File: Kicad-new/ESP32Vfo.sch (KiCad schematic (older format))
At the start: 63 parts, among them J1 ILI9341, J2 5V, J3 Jtag, J4 I2C, J6 I2C, J7 Encoders, J8 Encoders, J9 Analog in 3-6, SW1 SW_Push, SW2 SW_Push, U1 LM1117-3.3, U2 ESP32-WROOM-32D, U3 PCF8574A, U5 TCA9548APWR

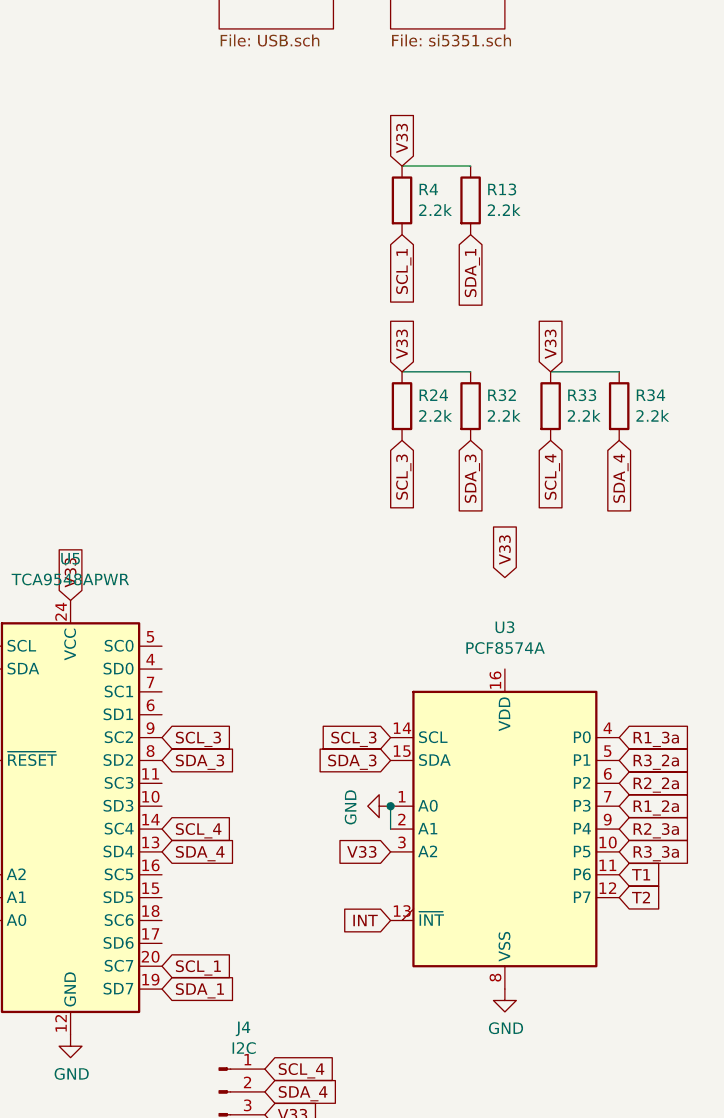
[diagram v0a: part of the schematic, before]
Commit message: new pcb
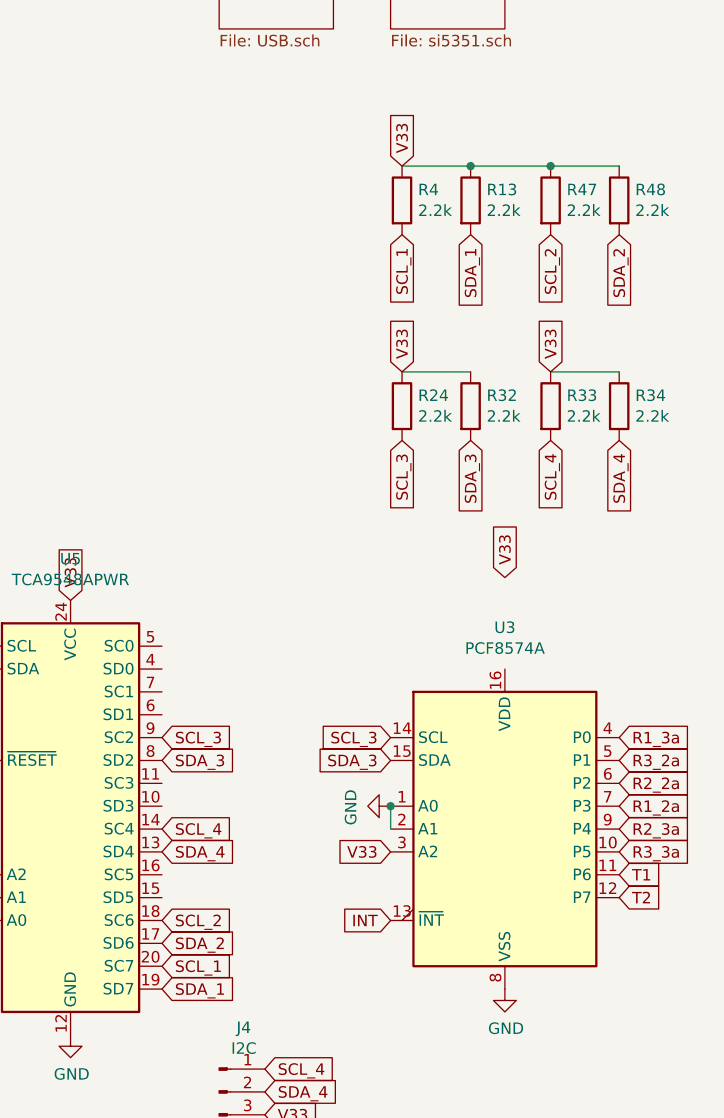
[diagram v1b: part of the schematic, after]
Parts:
- added R47, R48: 2.2k, Resistor_SMD:R_0805_2012Metric, symbol Device:R
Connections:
- net V33: now also R47.1, R48.1
- net SDA_2: now reaches U5.17 (SD6)
- net SDA_2: now also R48.2
- net SCL_2: now reaches U5.18 (SC6)
- net SCL_2: now also R47.2
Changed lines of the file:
@@
 Wire Wire Line
 	2050 1800 2300 1800
+Text GLabel 8850 5050 2    50   Input ~ 0
+SCL_2
+Text GLabel 8850 5150 2    50   Input ~ 0
+SDA_2
+$Comp
+L Device:R R?
+U 1 1 6169519F
+P 10550 1900
+AR Path="/614F5619/6169519F" Ref="R?"  Part="1"
+AR Path="/61506CC0/6169519F" Ref="R?"  Part="1"
+AR Path="/6169519F" Ref="R47"  Part="1"
+F 0 "R47" H 10620 1946 50  0000 L CNN
+F 1 "2.2k" H 10620 1855 50  0000 L CNN
+F 2 "Resistor_SMD:R_0805_2012Metric" V 10480 1900 50  0001 C CNN
+F 3 "~" H 10550 1900 50  0001 C CNN
+	1    10550 1900
+	1    0    0    -1
+$EndComp
+$Comp
+L Device:R R?
+U 1 1 616958E1
+P 10850 1900
+AR Path="/614F5619/616958E1" Ref="R?"  Part="1"
+AR Path="/61506CC0/616958E1" Ref="R?"  Part="1"
+AR Path="/616958E1" Ref="R48"  Part="1"
+F 0 "R48" H 10920 1946 50  0000 L CNN
+F 1 "2.2k" H 10920 1855 50  0000 L CNN
+F 2 "Resistor_SMD:R_0805_2012Metric" V 10780 1900 50  0001 C CNN
+F 3 "~" H 10850 1900 50  0001 C CNN
+	1    10850 1900
+	1    0    0    -1
+$EndComp
+Text GLabel 10550 2050 3    50   Input ~ 0
+SCL_2
+Text GLabel 10850 2050 3    50   Input ~ 0
+SDA_2
+Wire Wire Line
+	10200 1750 10550 1750
+Connection ~ 10200 1750
+Connection ~ 10550 1750
+Wire Wire Line
+	10550 1750 10850 1750
 $EndSCHEMATC

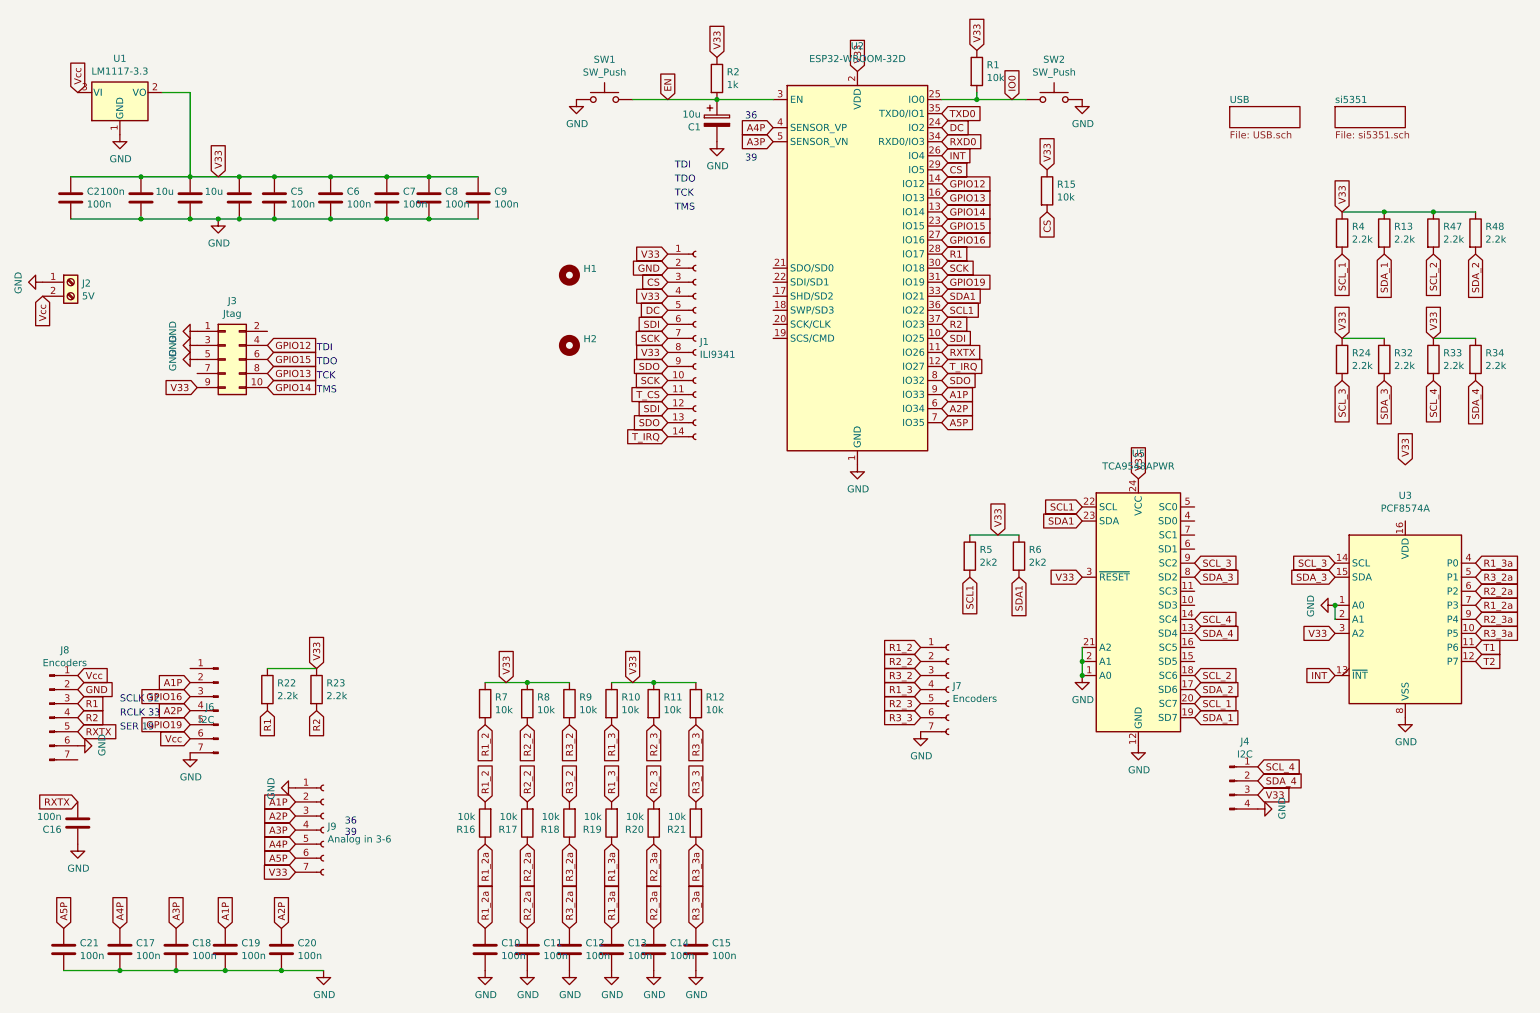
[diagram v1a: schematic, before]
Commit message: update pcb
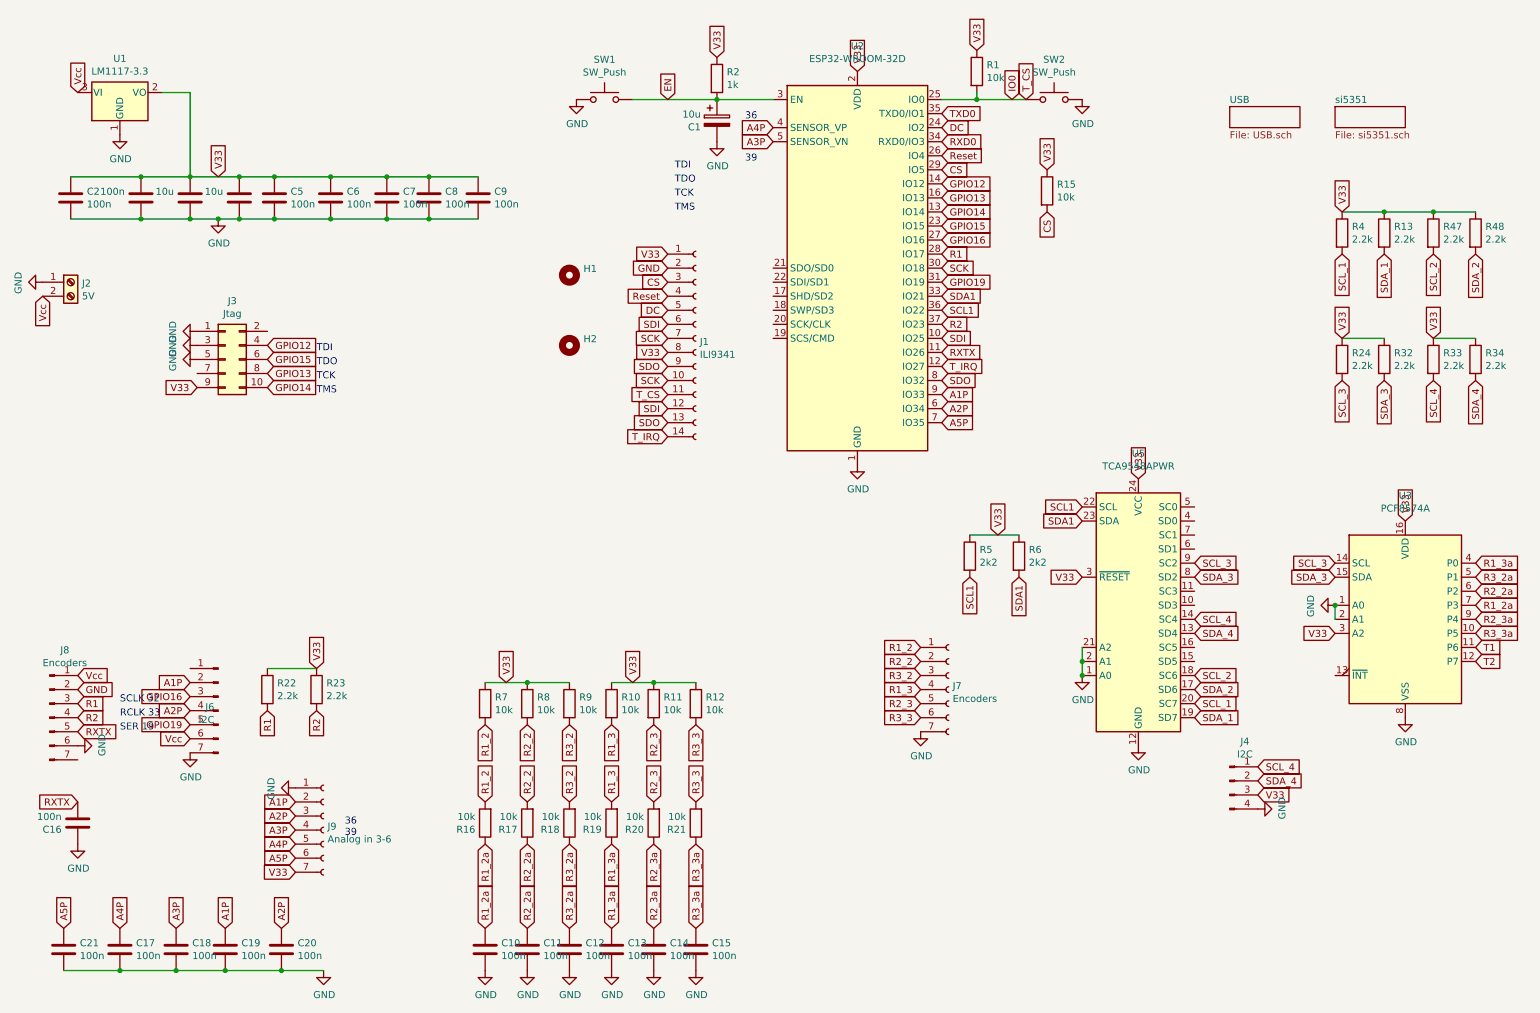
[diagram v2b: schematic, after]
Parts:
- SW1, SW2: footprint ESP32_TouchDown_lib:TS-1088R-02526 -> ESP32VFO:TS-1088R-02526
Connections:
- net T_CS is gone; now on net IO0: J1.11 (Pin_11)
- net V33: now also U3.16 (VDD); no longer J1.4 (Pin_4)
- net INT: no longer names the net of U3.13 (~INT~)
- net INT: no longer U2.26 (IO4)
- new net Reset: J1.4 (Pin_4), U2.26 (IO4)
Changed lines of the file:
@@
 	1    0    0    -1
 $EndComp
-Text GLabel 10350 3550 1    50   Input ~ 0
+Text GLabel 10350 3950 1    50   Input ~ 0
 V33
 Text GLabel 7050 2450 2    50   Input ~ 0
@@
 F 0 "SW1" H 4650 1235 50  0000 C CNN
 F 1 "SW_Push" H 4650 1144 50  0000 C CNN
-F 2 "ESP32_TouchDown_lib:TS-1088R-02526" H 4650 1150 50  0001 C CNN
+F 2 "ESP32VFO:TS-1088R-02526" H 4650 1150 50  0001 C CNN
 F 3 "~" H 4650 1150 50  0001 C CNN
 	1    4650 950
@@
 F 0 "SW2" H 7850 1235 50  0000 C CNN
 F 1 "SW_Push" H 7850 1144 50  0000 C CNN
-F 2 "ESP32_TouchDown_lib:TS-1088R-02526" H 7850 1150 50  0001 C CNN
+F 2 "ESP32VFO:TS-1088R-02526" H 7850 1150 50  0001 C CNN
 F 3 "~" H 7850 1150 50  0001 C CNN
 	1    7850 950
@@
 SDI
 Text GLabel 5100 2350 0    50   Input ~ 0
-V33
+Reset
 Text GLabel 5100 3250 0    50   Input ~ 0
 SDO
@@
 Text GLabel 5100 2750 0    50   Input ~ 0
 V33
-Text GLabel 9850 5050 0    50   Input ~ 0
-INT
-Text GLabel 7050 1350 2    50   Input ~ 0
-INT
 Text GLabel 800  6850 1    50   Input ~ 0
 A5P
@@
 Wire Wire Line
 	10550 1750 10850 1750
+Text GLabel 7650 950  1    50   Input ~ 0
+T_CS
+Text GLabel 7050 1350 2    50   Input ~ 0
+Reset
 $EndSCHEMATC
